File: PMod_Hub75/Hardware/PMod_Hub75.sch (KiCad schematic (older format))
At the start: 5 parts

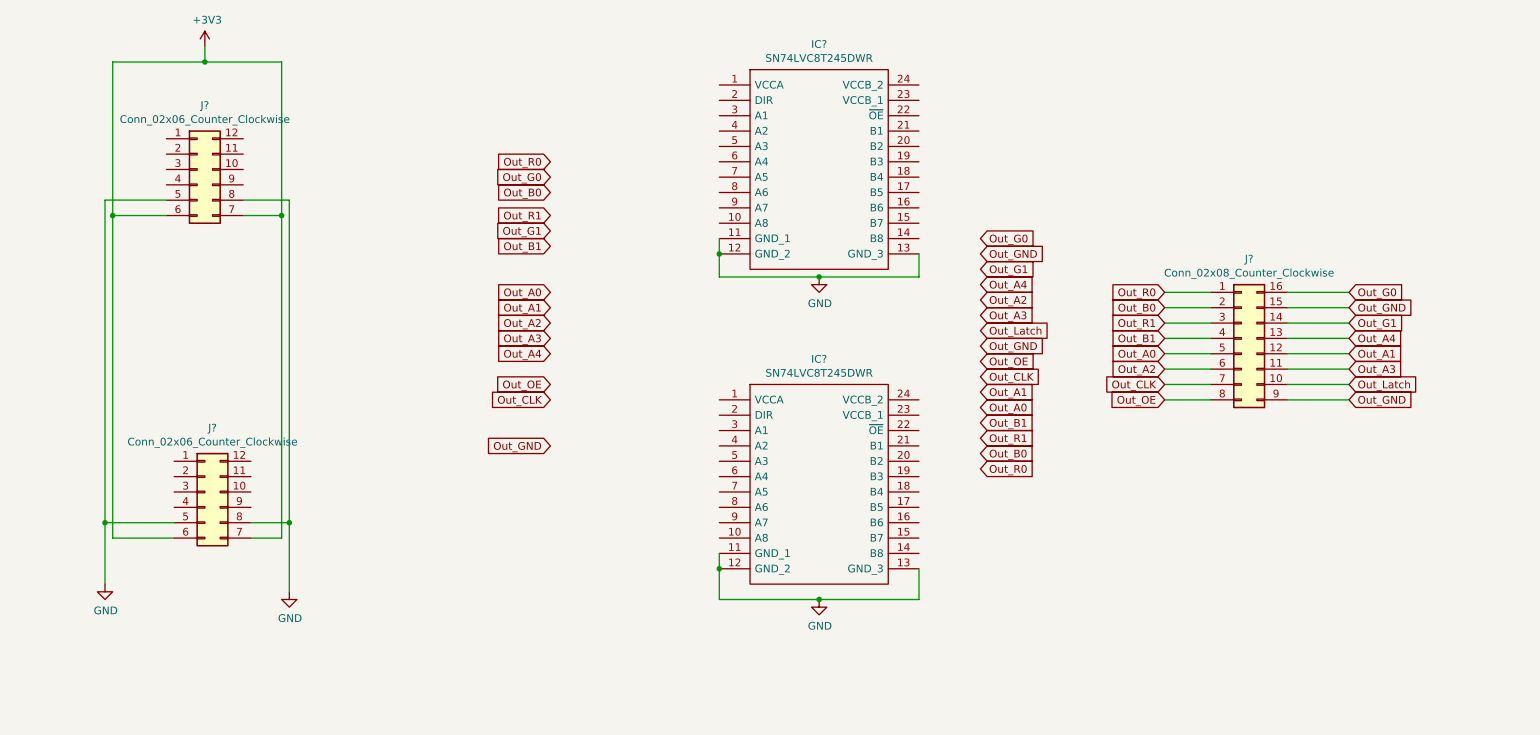
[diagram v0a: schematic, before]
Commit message: Add PMod connector pinout
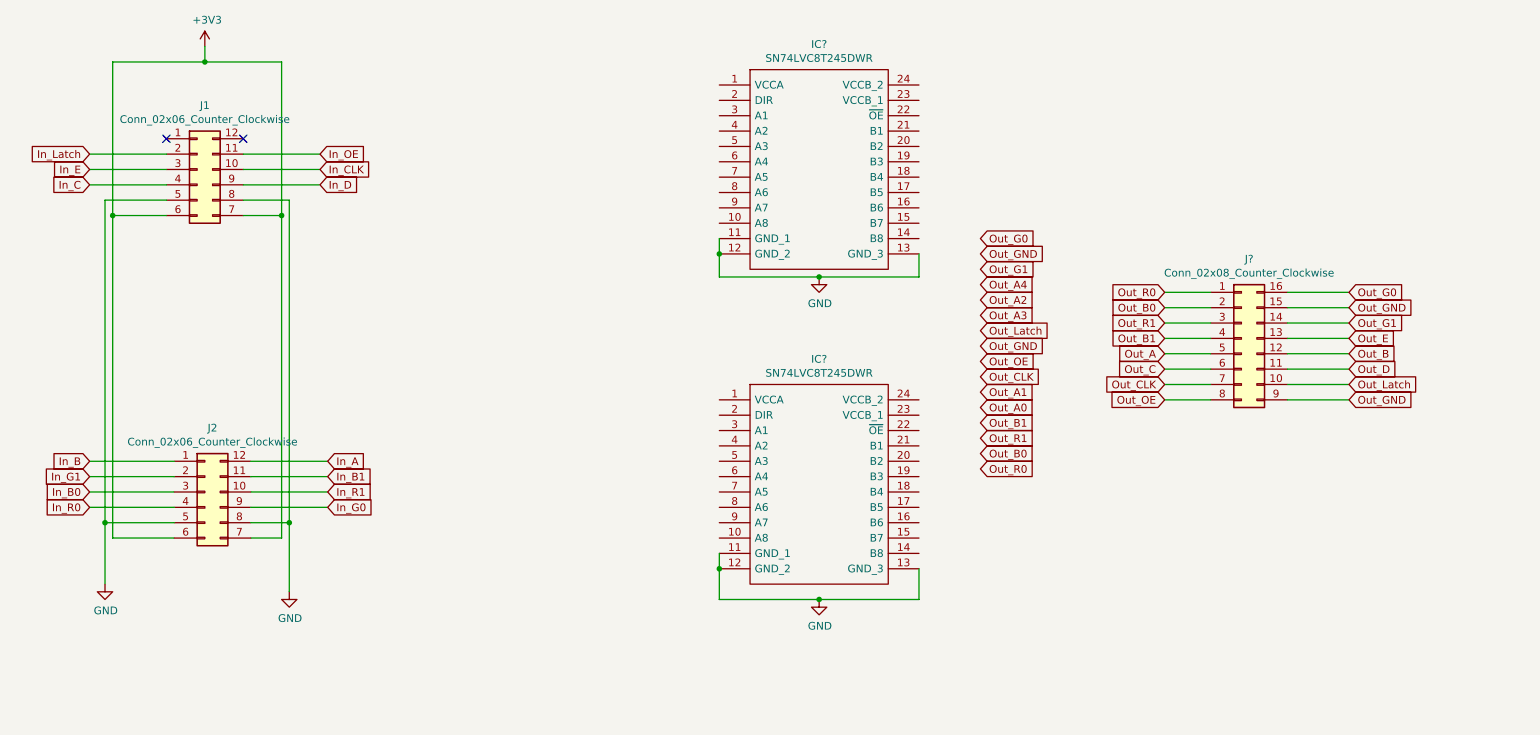
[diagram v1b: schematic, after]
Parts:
- J1, J2: renamed from J?; footprint (none) -> Connector_PinHeader_2.54mm:PinHeader_2x08_P2.54mm_Vertical
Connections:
- net Out_A0: no longer J?.5 (Pin_5)
- net Out_A1: no longer J?.12 (Pin_12)
- net Out_A2: no longer J?.6 (Pin_6)
- net Out_A3: no longer J?.11 (Pin_11)
- net Out_A4: no longer J?.13 (Pin_13)
- net In_CLK: now reaches J1.10 (Pin_10)
- net In_OE: now reaches J1.11 (Pin_11)
- net In_Latch: now reaches J1.2 (Pin_2)
- net In_E: now reaches J1.3 (Pin_3)
- net In_C: now reaches J1.4 (Pin_4)
- net In_D: now reaches J1.9 (Pin_9)
- net In_B: now reaches J2.1 (Pin_1)
- net In_R1: now reaches J2.10 (Pin_10)
- net In_B1: now reaches J2.11 (Pin_11)
- net In_A: now reaches J2.12 (Pin_12)
- net In_G1: now reaches J2.2 (Pin_2)
- net In_B0: now reaches J2.3 (Pin_3)
- net In_R0: now reaches J2.4 (Pin_4)
- net In_G0: now reaches J2.9 (Pin_9)
- new net Out_A: J?.5 (Pin_5)
- new net Out_B: J?.12 (Pin_12)
- new net Out_C: J?.6 (Pin_6)
- new net Out_D: J?.11 (Pin_11)
- new net Out_E: J?.13 (Pin_13)
- no-connect marks 0 -> 2
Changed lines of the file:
@@
 $EndComp
 $Comp
-L Connector_Generic:Conn_02x06_Counter_Clockwise J?
+L Connector_Generic:Conn_02x06_Counter_Clockwise J1
 U 1 1 61C3C515
 P 2200 2600
-F 0 "J?" H 2250 3017 50  0000 C CNN
+F 0 "J1" H 2250 3017 50  0000 C CNN
 F 1 "Conn_02x06_Counter_Clockwise" H 2250 2926 50  0000 C CNN
-F 2 "" H 2200 2600 50  0001 C CNN
+F 2 "Connector_PinHeader_2.54mm:PinHeader_2x08_P2.54mm_Vertical" H 2200 2600 50  0001 C CNN
 F 3 "~" H 2200 2600 50  0001 C CNN
 	1    2200 2600
@@
 $EndComp
 $Comp
-L Connector_Generic:Conn_02x06_Counter_Clockwise J?
+L Connector_Generic:Conn_02x06_Counter_Clockwise J2
 U 1 1 61C3D51F
 P 2250 4700
-F 0 "J?" H 2300 5117 50  0000 C CNN
+F 0 "J2" H 2300 5117 50  0000 C CNN
 F 1 "Conn_02x06_Counter_Clockwise" H 2300 5026 50  0000 C CNN
-F 2 "" H 2250 4700 50  0001 C CNN
+F 2 "Connector_PinHeader_2.54mm:PinHeader_2x08_P2.54mm_Vertical" H 2250 4700 50  0001 C CNN
 F 3 "~" H 2250 4700 50  0001 C CNN
 	1    2250 4700
@@
 Out_B1
 Text GLabel 8500 3800 0    50   Input ~ 0
-Out_A0
+Out_A
 Text GLabel 8500 3900 0    50   Input ~ 0
-Out_A2
+Out_C
 Text GLabel 8500 4000 0    50   Input ~ 0
 Out_CLK
@@
 Out_Latch
 Text GLabel 9700 3900 2    50   Input ~ 0
-Out_A3
+Out_D
 Text GLabel 9700 3800 2    50   Input ~ 0
-Out_A1
+Out_B
 Text GLabel 9700 3700 2    50   Input ~ 0
-Out_A4
+Out_E
 Text GLabel 9700 3600 2    50   Input ~ 0
 Out_G1
@@
 Text GLabel 7300 3050 2    50   Input ~ 0
 Out_G0
-Text GLabel 4500 2550 0    50   Input ~ 0
-Out_R0
-Text GLabel 4500 2750 0    50   Input ~ 0
-Out_B0
-Text GLabel 4500 2900 0    50   Input ~ 0
-Out_R1
-Text GLabel 4500 3100 0    50   Input ~ 0
-Out_B1
-Text GLabel 4500 3400 0    50   Input ~ 0
-Out_A0
-Text GLabel 4500 3500 0    50   Input ~ 0
-Out_A1
-Text GLabel 4500 4100 0    50   Input ~ 0
-Out_CLK
-Text GLabel 4500 4000 0    50   Input ~ 0
-Out_OE
-Text GLabel 4500 4400 0    50   Input ~ 0
-Out_GND
-Text GLabel 4500 3700 0    50   Input ~ 0
-Out_A3
-Text GLabel 4500 3600 0    50   Input ~ 0
-Out_A2
-Text GLabel 4500 3800 0    50   Input ~ 0
-Out_A4
-Text GLabel 4500 3000 0    50   Input ~ 0
-Out_G1
-Text GLabel 4500 2650 0    50   Input ~ 0
-Out_G0
+Text GLabel 1500 4800 0    50   Input ~ 0
+In_R0
+Text GLabel 1500 4700 0    50   Input ~ 0
+In_B0
+Text GLabel 3050 4600 2    50   Input ~ 0
+In_B1
+Text GLabel 3050 4500 2    50   Input ~ 0
+In_A
+Text GLabel 1500 4500 0    50   Input ~ 0
+In_B
+Text GLabel 3000 2600 2    50   Input ~ 0
+In_CLK
+Text GLabel 3000 2500 2    50   Input ~ 0
+In_OE
+Text GLabel 3000 2700 2    50   Input ~ 0
+In_D
+Text GLabel 1500 2700 0    50   Input ~ 0
+In_C
+Text GLabel 1500 2600 0    50   Input ~ 0
+In_E
+Text GLabel 1500 4600 0    50   Input ~ 0
+In_G1
+Text GLabel 3050 4800 2    50   Input ~ 0
+In_G0
+Text GLabel 3050 4700 2    50   Input ~ 0
+In_R1
+Text GLabel 1500 2500 0    50   Input ~ 0
+In_Latch
+NoConn ~ 2000 2400
+NoConn ~ 2500 2400
+Wire Wire Line
+	2500 2500 3000 2500
+Wire Wire Line
+	3000 2600 2500 2600
+Wire Wire Line
+	2500 2700 3000 2700
+Wire Wire Line
+	2000 2700 1500 2700
+Wire Wire Line
+	1500 2600 2000 2600
+Wire Wire Line
+	2000 2500 1500 2500
+Wire Wire Line
+	1500 4500 2050 4500
+Wire Wire Line
+	1500 4600 2050 4600
+Wire Wire Line
+	2550 4500 3050 4500
+Wire Wire Line
+	3050 4600 2550 4600
+Wire Wire Line
+	2550 4700 3050 4700
+Wire Wire Line
+	3050 4800 2550 4800
+Wire Wire Line
+	2050 4700 1500 4700
+Wire Wire Line
+	1500 4800 2050 4800
 $EndSCHEMATC

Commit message: finish schematic and place main components on PCB
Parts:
- added C1, C2, C3, C4: 100n, Capacitor_SMD:C_0603_1608Metric, symbol Device:C
- added R1, R2, R3, R4: 10k, Resistor_SMD:R_0603_1608Metric, symbol Device:R
- J1, J2: footprint Connector_PinHeader_2.54mm:PinHeader_2x08_P2.54mm_Vertical -> Connector_PinHeader_2.54mm:PinHeader_2x06_P2.54mm_Vertical; symbol Connector_Generic:Conn_02x06_Counter_Clockwise -> Connector_Generic:Conn_02x06_Odd_Even
- J3: renamed from J?; footprint (none) -> Connector_PinHeader_2.54mm:PinHeader_2x08_P2.54mm_Vertical; symbol Connector_Generic:Conn_02x08_Counter_Clockwise -> Connector_Generic:Conn_02x08_Odd_Even
- gave numbers to parts that had none: 2
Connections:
- net +3V3: now also IC1.1 (VCCA), IC2.1 (VCCA), J1.11 (Pin_11), J1.12 (Pin_12), J2.11 (Pin_11), J2.12 (Pin_12), C1.1, C2.1, R1.1, R2.1; no longer J1.6 (Pin_6), J1.7 (Pin_7), J2.6 (Pin_6), J2.7 (Pin_7)
- net GND: now also IC1.3 (A1), IC1.4 (A2), J1.10 (Pin_10), J1.9 (Pin_9), J2.10 (Pin_10), J2.9 (Pin_9), C1.2, C2.2, C3.1, C4.1, R3.2, R4.2; no longer J1.5 (Pin_5), J1.8 (Pin_8), J2.5 (Pin_5), J2.8 (Pin_8)
- net In_A: now also IC2.4 (A2), J2.2 (Pin_2); no longer J2.12 (Pin_12)
- net In_B: now also IC2.3 (A1)
- net In_B0: now also IC2.8 (A6), J2.5 (Pin_5); no longer J2.3 (Pin_3)
- net In_B1: now also IC2.5 (A3), J2.4 (Pin_4); no longer J2.11 (Pin_11)
- net In_C: now also IC1.10 (A8), J1.7 (Pin_7); no longer J1.4 (Pin_4)
- net In_CLK: now also IC1.7 (A5), J1.6 (Pin_6); no longer J1.10 (Pin_10)
- net In_D: now also IC1.9 (A7), J1.8 (Pin_8); no longer J1.9 (Pin_9)
- net In_E: now also IC1.8 (A6), J1.5 (Pin_5); no longer J1.3 (Pin_3)
- net In_G0: now also IC2.9 (A7), J2.8 (Pin_8); no longer J2.9 (Pin_9)
- net In_G1: now also IC2.6 (A4), J2.3 (Pin_3); no longer J2.2 (Pin_2)
- net In_Latch: now also IC1.5 (A3), J1.3 (Pin_3); no longer J1.2 (Pin_2)
- net In_OE: now also IC1.6 (A4), J1.4 (Pin_4); no longer J1.11 (Pin_11)
- net In_R0: now also IC2.10 (A8), J2.7 (Pin_7); no longer J2.4 (Pin_4)
- net In_R1: now also IC2.7 (A5), J2.6 (Pin_6); no longer J2.10 (Pin_10)
- net Out_A: now also IC2.20 (B2), J3.9 (Pin_9); no longer J3.5 (Pin_5)
- net Out_B: now also IC2.21 (B1), J3.10 (Pin_10); no longer J3.12 (Pin_12)
- net Out_B0: now also IC2.15 (B7), J3.3 (Pin_3); no longer J3.2 (Pin_2)
- net Out_B1: now also IC2.18 (B4), J3.7 (Pin_7); no longer J3.4 (Pin_4)
- net Out_C: now also IC1.14 (B8), J3.11 (Pin_11); no longer J3.6 (Pin_6)
- net Out_CLK: now also IC1.17 (B5), J3.13 (Pin_13); no longer J3.7 (Pin_7)
- net Out_D: now also IC1.15 (B7), J3.12 (Pin_12); no longer J3.11 (Pin_11)
- net Out_E: now also IC1.16 (B6), J3.8 (Pin_8); no longer J3.13 (Pin_13)
- net Out_G0: now also IC2.16 (B6), J3.2 (Pin_2); no longer J3.16 (Pin_16)
- net Out_G1: now also IC2.19 (B3), J3.6 (Pin_6); no longer J3.14 (Pin_14)
- net Out_GND: now also J3.16 (Pin_16), J3.4 (Pin_4); no longer J3.15 (Pin_15), J3.9 (Pin_9)
- net Out_Latch: now also IC1.19 (B3), J3.14 (Pin_14); no longer J3.10 (Pin_10)
- net Out_OE: now also IC1.18 (B4), J3.15 (Pin_15); no longer J3.8 (Pin_8)
- net Out_R0: now also IC2.14 (B8)
- net Out_R1: now also IC2.17 (B5), J3.5 (Pin_5); no longer J3.3 (Pin_3)
- net at IC1.2 (DIR): now also R1.2
- net at IC1.22 (~OE): now also R3.1
- net VCC: now reaches IC1.23 (VCCB_1)
- net VCC: now also IC1.24 (VCCB_2), IC2.23 (VCCB_1), IC2.24 (VCCB_2), C3.2, C4.2
- net at IC2.2 (DIR): now also R2.2
- net at IC2.22 (~OE): now also R4.1
- no-connect marks 2 -> 4
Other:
- moved on the sheet: J3

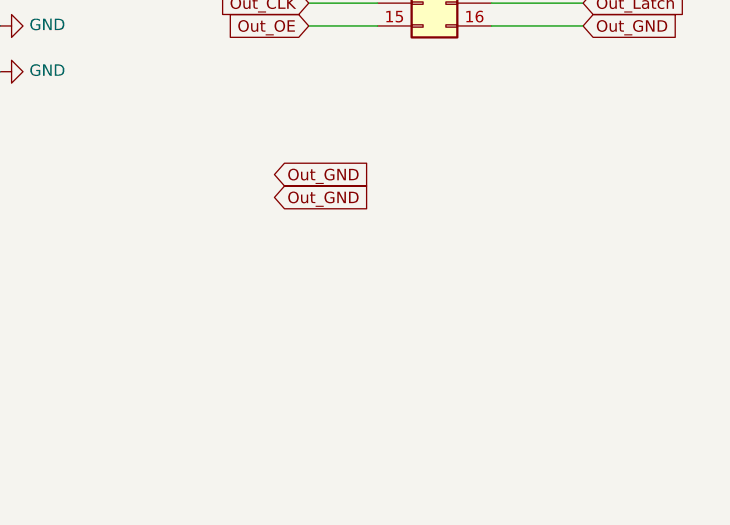
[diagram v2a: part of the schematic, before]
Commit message: Update scematic with 3v3 output level and shared ground output
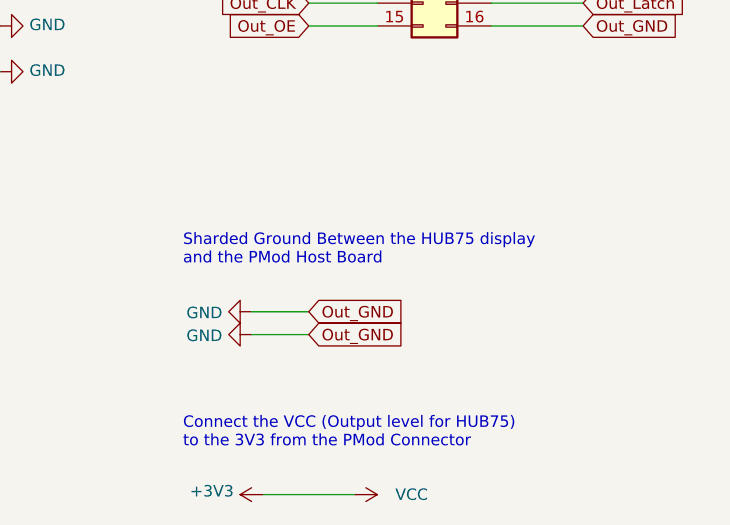
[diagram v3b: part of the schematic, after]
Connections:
- net Out_GND is gone; now on net GND: J3.16 (Pin_16), J3.4 (Pin_4)
- net VCC is gone; now on net +3V3: C3.2, C4.2, IC1.23 (VCCB_1), IC1.24 (VCCB_2), IC2.23 (VCCB_1), IC2.24 (VCCB_2)
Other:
- note added: "Connect the VCC (Output level for HUB75)\nto the 3V3 from the PMod Connector"
- note added: "Sharded Ground Between the HUB75 display \nand the PMod Host Board"
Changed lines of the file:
@@
 Text GLabel 7200 2650 2    50   Input ~ 0
 Out_OE
-Text GLabel 8950 4850 2    50   Input ~ 0
+Text GLabel 9100 5450 2    50   Input ~ 0
 Out_GND
 Text GLabel 7200 2550 2    50   Input ~ 0
@@
 Text GLabel 7200 4600 2    50   Input ~ 0
 Out_G1
-Text GLabel 8950 4750 2    50   Input ~ 0
+Text GLabel 9100 5350 2    50   Input ~ 0
 Out_GND
 Text GLabel 7200 4900 2    50   Input ~ 0
@@
 NoConn ~ 6900 2350
 NoConn ~ 6900 2450
+$Comp
+L power:GND #PWR?
+U 1 1 61D10CA9
+P 8850 5350
+F 0 "#PWR?" H 8850 5100 50  0001 C CNN
+F 1 "GND" V 8855 5222 50  0000 R CNN
+F 2 "" H 8850 5350 50  0001 C CNN
+F 3 "" H 8850 5350 50  0001 C CNN
+	1    8850 5350
+	0    1    1    0
+$EndComp
+$Comp
+L power:GND #PWR?
+U 1 1 61D10CAF
+P 8850 5450
+F 0 "#PWR?" H 8850 5200 50  0001 C CNN
+F 1 "GND" V 8855 5322 50  0000 R CNN
+F 2 "" H 8850 5450 50  0001 C CNN
+F 3 "" H 8850 5450 50  0001 C CNN
+	1    8850 5450
+	0    1    1    0
+$EndComp
+Wire Wire Line
+	9100 5350 8850 5350
+Wire Wire Line
+	8850 5450 9100 5450
+$Comp
+L power:VCC #PWR?
+U 1 1 61D2486A
+P 9300 6150
+F 0 "#PWR?" H 9300 6000 50  0001 C CNN
+F 1 "VCC" V 9300 6400 50  0000 C CNN
+F 2 "" H 9300 6150 50  0001 C CNN
+F 3 "" H 9300 6150 50  0001 C CNN
+	1    9300 6150
+	0    1    1    0
+$EndComp
+$Comp
+L power:+3V3 #PWR?
+U 1 1 61D29B56
+P 8900 6150
+F 0 "#PWR?" H 8900 6000 50  0001 C CNN
+F 1 "+3V3" V 8915 6278 50  0000 L CNN
+F 2 "" H 8900 6150 50  0001 C CNN
+F 3 "" H 8900 6150 50  0001 C CNN
+	1    8900 6150
+	0    -1   -1   0
+$EndComp
+Wire Wire Line
+	8900 6150 9300 6150
+Text Notes 8550 5950 0    50   ~ 0
+Connect the VCC (Output level for HUB75)\nto the 3V3 from the PMod Connector
+Text Notes 8550 5150 0    50   ~ 0
+Sharded Ground Between the HUB75 display \nand the PMod Host Board
 $EndSCHEMATC

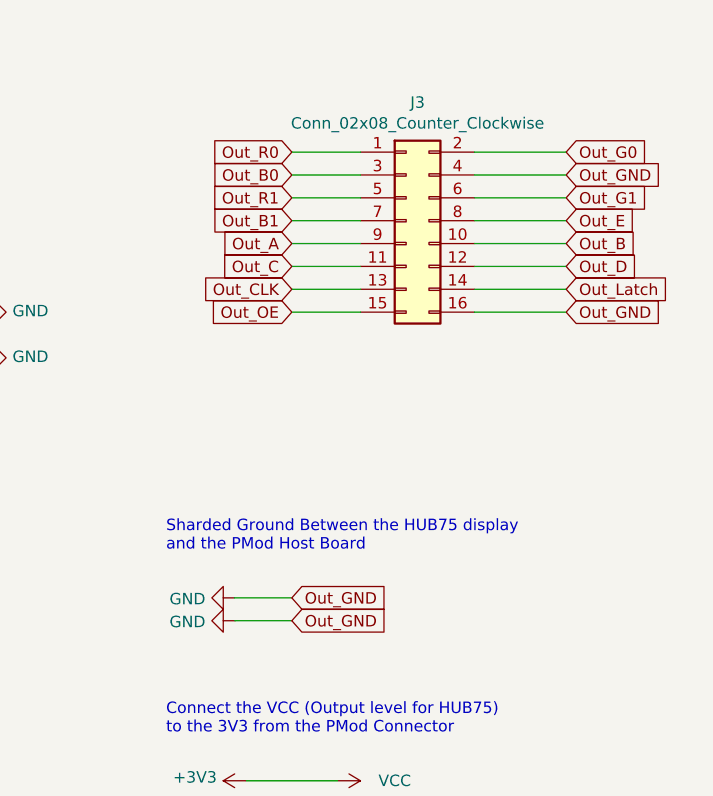
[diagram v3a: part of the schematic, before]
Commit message: Update the routing of 3v3 and GND
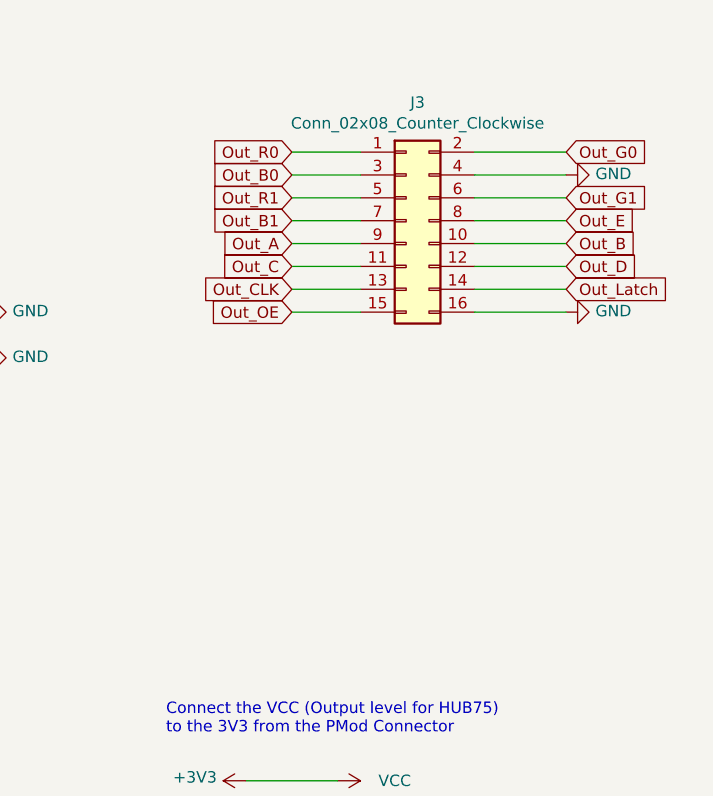
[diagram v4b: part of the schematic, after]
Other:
- note removed: "Sharded Ground Between the HUB75 display \nand the PMod Host Board"
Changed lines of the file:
@@
 Text GLabel 9100 4100 0    50   Input ~ 0
 Out_OE
-Text GLabel 10300 4100 2    50   Input ~ 0
-Out_GND
 Text GLabel 10300 4000 2    50   Input ~ 0
 Out_Latch
@@
 Text GLabel 10300 3600 2    50   Input ~ 0
 Out_G1
-Text GLabel 10300 3500 2    50   Input ~ 0
-Out_GND
 Text GLabel 10300 3400 2    50   Input ~ 0
 Out_G0
@@
 Text GLabel 7200 2650 2    50   Input ~ 0
 Out_OE
-Text GLabel 9100 5450 2    50   Input ~ 0
-Out_GND
 Text GLabel 7200 2550 2    50   Input ~ 0
 Out_Latch
@@
 Text GLabel 7200 4600 2    50   Input ~ 0
 Out_G1
-Text GLabel 9100 5350 2    50   Input ~ 0
-Out_GND
 Text GLabel 7200 4900 2    50   Input ~ 0
 Out_G0
@@
 NoConn ~ 6900 2450
 $Comp
-L power:GND #PWR?
-U 1 1 61D10CA9
-P 8850 5350
-F 0 "#PWR?" H 8850 5100 50  0001 C CNN
-F 1 "GND" V 8855 5222 50  0000 R CNN
-F 2 "" H 8850 5350 50  0001 C CNN
-F 3 "" H 8850 5350 50  0001 C CNN
-	1    8850 5350
-	0    1    1    0
-$EndComp
-$Comp
-L power:GND #PWR?
-U 1 1 61D10CAF
-P 8850 5450
-F 0 "#PWR?" H 8850 5200 50  0001 C CNN
-F 1 "GND" V 8855 5322 50  0000 R CNN
-F 2 "" H 8850 5450 50  0001 C CNN
-F 3 "" H 8850 5450 50  0001 C CNN
-	1    8850 5450
-	0    1    1    0
-$EndComp
-Wire Wire Line
-	9100 5350 8850 5350
-Wire Wire Line
-	8850 5450 9100 5450
-$Comp
-L power:VCC #PWR?
+L power:VCC #PWR0120
 U 1 1 61D2486A
 P 9300 6150
-F 0 "#PWR?" H 9300 6000 50  0001 C CNN
+F 0 "#PWR0120" H 9300 6000 50  0001 C CNN
 F 1 "VCC" V 9300 6400 50  0000 C CNN
 F 2 "" H 9300 6150 50  0001 C CNN
@@
 $EndComp
 $Comp
-L power:+3V3 #PWR?
+L power:+3V3 #PWR0121
 U 1 1 61D29B56
 P 8900 6150
-F 0 "#PWR?" H 8900 6000 50  0001 C CNN
+F 0 "#PWR0121" H 8900 6000 50  0001 C CNN
 F 1 "+3V3" V 8915 6278 50  0000 L CNN
 F 2 "" H 8900 6150 50  0001 C CNN
@@
 Text Notes 8550 5950 0    50   ~ 0
 Connect the VCC (Output level for HUB75)\nto the 3V3 from the PMod Connector
-Text Notes 8550 5150 0    50   ~ 0
-Sharded Ground Between the HUB75 display \nand the PMod Host Board
+$Comp
+L power:GND #PWR?
+U 1 1 61D511B2
+P 10300 4100
+F 0 "#PWR?" H 10300 3850 50  0001 C CNN
+F 1 "GND" V 10305 3972 50  0000 R CNN
+F 2 "" H 10300 4100 50  0001 C CNN
+F 3 "" H 10300 4100 50  0001 C CNN
+	1    10300 4100
+	0    -1   -1   0
+$EndComp
+$Comp
+L power:GND #PWR?
+U 1 1 61D511B8
+P 10300 3500
+F 0 "#PWR?" H 10300 3250 50  0001 C CNN
+F 1 "GND" V 10305 3372 50  0000 R CNN
+F 2 "" H 10300 3500 50  0001 C CNN
+F 3 "" H 10300 3500 50  0001 C CNN
+	1    10300 3500
+	0    -1   -1   0
+$EndComp
 $EndSCHEMATC
